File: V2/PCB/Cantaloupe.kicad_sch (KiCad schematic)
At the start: 124 parts, among them J1 USB_In, J2 OLED, J3 Link, J4 Debug, J5 Trackball, J6 Trackpad, Q1 2N7002, Q2 AO3401A, SW1 MX, SW10 MX, SW11 MX, SW12 MX, SW13 MX, SW14 MX, SW15 MX, SW16 MX, SW17 MX, SW18 MX, SW19 MX, SW2 MX, SW20 MX, SW21 MX, SW22 MX, SW23 MX, SW24 MX, SW25 MX, SW26 MX, SW27 MX, SW28 MX, SW29 MX, SW3 MX, SW30 MX, SW31 Encoder, SW32 MX, SW4 MX, SW5 MX, SW6 MX, SW7 MX, SW8 MX, SW9 MX, U1 STM32F4x1CxUx, U2 SRV0504, U3 SRV0504, U4 XC6206P332MR, U5 LMV321, Y1 8MHz

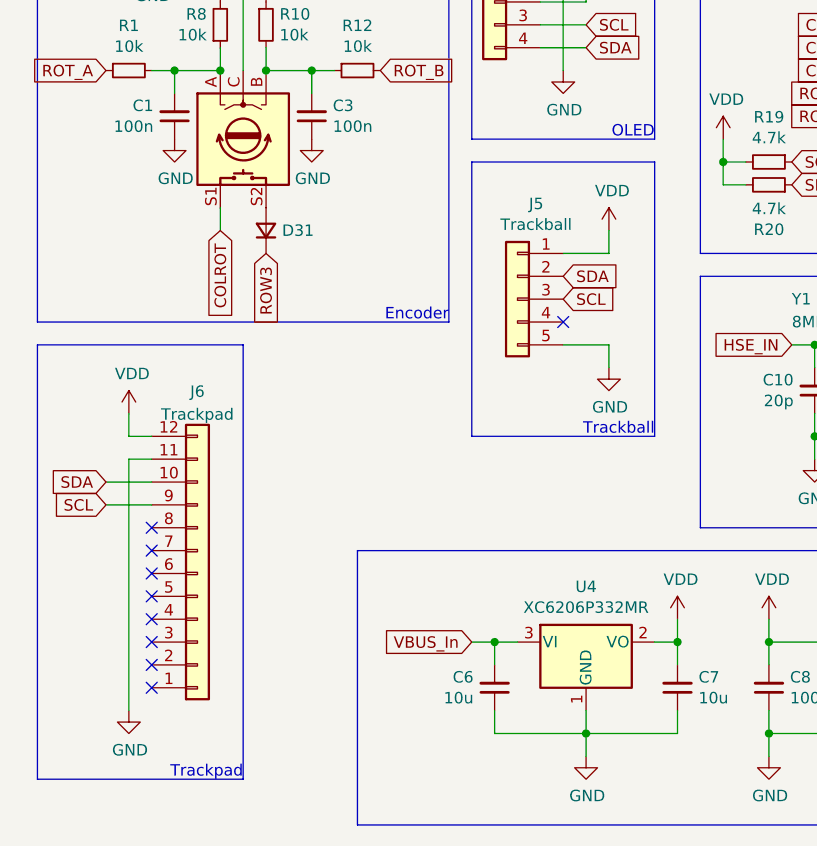
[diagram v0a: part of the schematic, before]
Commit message: Update to V2.1
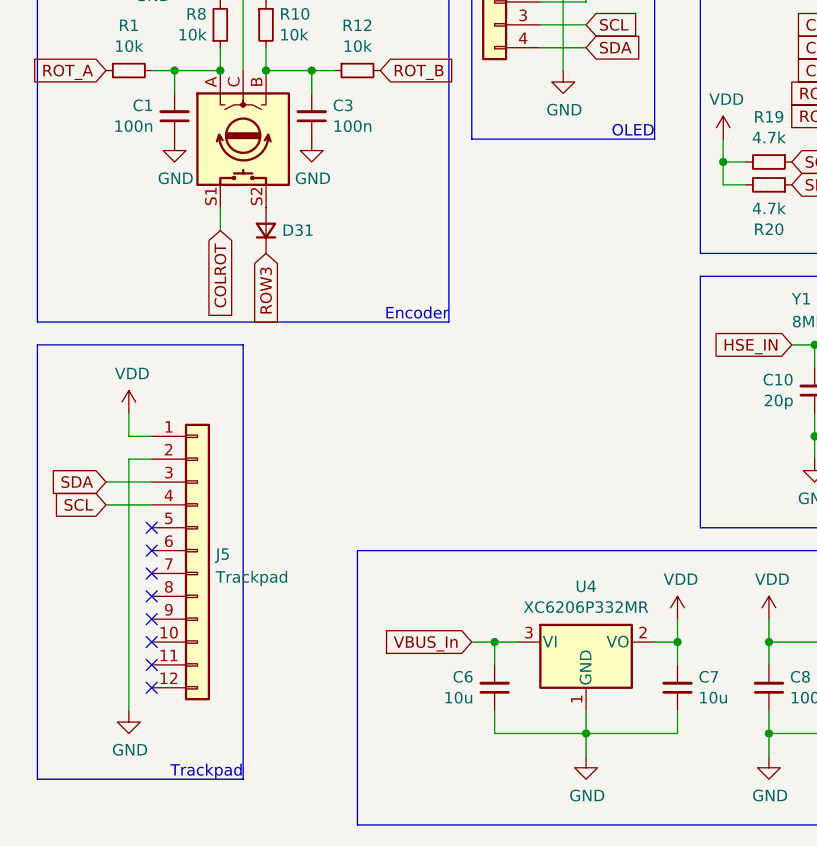
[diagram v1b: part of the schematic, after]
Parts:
- removed J5: Trackball, Ariamelon:pimoroni_trackball_flippable, symbol Connector_Generic:Conn_01x05
- J5: renamed from J6; footprint Ariamelon:FPC-SMD_FPC05012-09200-.5mm-rev -> Connector_FFC-FPC:Hirose_FH12-12S-0.5SH_1x12-1MP_P0.50mm_Horizontal
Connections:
- net GND: now also J5.2 (Pin_2); no longer J5.11 (Pin_11)
- net SCL: now also J5.4 (Pin_4); no longer J5.9 (Pin_9)
- net SDA: now also J5.3 (Pin_3); no longer J5.10 (Pin_10)
- net VDD: now also J5.1 (Pin_1); no longer J5.12 (Pin_12)
- no-connect marks 27 -> 26
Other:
- note removed: "Trackball"
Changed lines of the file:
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@@
   (no_connect (at 30.48 160.02))
   (no_connect (at 109.22 58.42))
-  (no_connect (at 76.2 121.92))
   (no_connect (at 30.48 147.32))
   (no_connect (at 190.5 55.88))
@@
     (stroke (width 0) (type default) (color 0 0 0 0))
   )
-  (wire (pts (xy 81.28 114.3) (xy 81.28 111.76))
-    (stroke (width 0) (type default) (color 0 0 0 0))
-  )
   (polyline (pts (xy 200.66 15.24) (xy 200.66 71.12))
     (stroke (width 0) (type default) (color 0 0 0 0))
@@
     (stroke (width 0) (type default) (color 0 0 0 0))
   )
-  (polyline (pts (xy 86.36 104.14) (xy 66.04 104.14))
-    (stroke (width 0) (type default) (color 0 0 0 0))
-  )
   (wire (pts (xy 38.1 22.86) (xy 38.1 25.4))
     (stroke (width 0) (type default) (color 0 0 0 0))
@@
     (stroke (width 0) (type default) (color 0 0 0 0))
   )
-  (polyline (pts (xy 66.04 134.62) (xy 86.36 134.62))
-    (stroke (width 0) (type default) (color 0 0 0 0))
-  )
   (wire (pts (xy 129.54 165.1) (xy 129.54 167.64))
     (stroke (width 0) (type default) (color 0 0 0 0))
@@
     (stroke (width 0) (type default) (color 0 0 0 0))
   )
-  (wire (pts (xy 81.28 124.46) (xy 76.2 124.46))
-    (stroke (width 0) (type default) (color 0 0 0 0))
-  )
   (polyline (pts (xy 134.62 116.84) (xy 134.62 144.78))
     (stroke (width 0) (type default) (color 0 0 0 0))
@@
     (stroke (width 0) (type default) (color 0 0 0 0))
   )
-  (polyline (pts (xy 66.04 104.14) (xy 66.04 134.62))
-    (stroke (width 0) (type default) (color 0 0 0 0))
-  )
   (wire (pts (xy 60.96 35.56) (xy 58.42 35.56))
     (stroke (width 0) (type default) (color 0 0 0 0))
@@
     (stroke (width 0) (type default) (color 0 0 0 0))
   )
-  (polyline (pts (xy 86.36 134.62) (xy 86.36 104.14))
-    (stroke (width 0) (type default) (color 0 0 0 0))
-  )
   (wire (pts (xy 68.58 157.48) (xy 71.12 157.48))
     (stroke (width 0) (type default) (color 0 0 0 0))
@@
     (stroke (width 0) (type default) (color 0 0 0 0))
   )
-  (wire (pts (xy 81.28 127) (xy 81.28 124.46))
-    (stroke (width 0) (type default) (color 0 0 0 0))
-  )
   (wire (pts (xy 96.52 106.68) (xy 93.98 106.68))
     (stroke (width 0) (type default) (color 0 0 0 0))
@@
     (stroke (width 0) (type default) (color 0 0 0 0))
   )
-  (wire (pts (xy 76.2 114.3) (xy 81.28 114.3))
-    (stroke (width 0) (type default) (color 0 0 0 0))
-  )
   (wire (pts (xy 76.2 71.12) (xy 66.04 71.12))
     (stroke (width 0) (type default) (color 0 0 0 0))
@@
     (effects (font (size 1.27 1.27)) (justify right bottom))
   )
-  (text "Trackball" (at 86.36 134.62 180)
-    (effects (font (size 1.27 1.27)) (justify right bottom))
-  )
   (global_label "D-" (shape input) (at 170.18 91.44 180) (fields_autoplaced)
     (effects (font (size 1.27 1.27)) (justify right))
@@
     )
   )
-  (global_label "SCL" (shape input) (at 76.2 119.38 0) (fields_autoplaced)
-    (effects (font (size 1.27 1.27)) (justify left))
-    (property "Intersheet References" "${INTERSHEET_REFS}" (id 0) (at 0 0 0)
-      (effects (font (size 1.27 1.27)) hide)
-    )
-  )
   (global_label "ROW1" (shape input) (at 25.4 40.64 180) (fields_autoplaced)
     (effects (font (size 1.27 1.27)) (justify right))
@@
     )
   )
-  (global_label "SDA" (shape input) (at 76.2 116.84 0) (fields_autoplaced)
-    (effects (font (size 1.27 1.27)) (justify left))
-    (property "Intersheet References" "${INTERSHEET_REFS}" (id 0) (at 0 0 0)
-      (effects (font (size 1.27 1.27)) hide)
-    )
-  )
   (global_label "SDA" (shape input) (at 109.22 81.28 180) (fields_autoplaced)
     (effects (font (size 1.27 1.27)) (justify right))
@@
     (pin "1")
   )
-  (symbol (lib_id "Connector_Generic:Conn_01x05") (at 71.12 119.38 0) (mirror y) (unit 1)
-    (in_bom yes) (on_board yes)
-    (property "Reference" "J5" (id 0) (at 73.2028 108.7882 0))
-    (property "Value" "Trackball" (id 1) (at 73.2028 111.0996 0))
-    (property "Footprint" "Ariamelon:pimoroni_trackball_flippable" (id 2) (at 71.12 119.38 0)
-      (effects (font (size 1.27 1.27)) hide)
-    )
-    (property "Datasheet" "~" (id 3) (at 71.12 119.38 0)
-      (effects (font (size 1.27 1.27)) hide)
-    )
-    (pin "1")
-    (pin "2")
-    (pin "3")
-    (pin "4")
-    (pin "5")
-  )
-  (symbol (lib_id "power:VDD") (at 81.28 111.76 0) (unit 1)
-    (in_bom yes) (on_board yes)
-    (property "Reference" "#PWR0130" (id 0) (at 81.28 115.57 0)
-      (effects (font (size 1.27 1.27)) hide)
-    )
-    (property "Value" "VDD" (id 1) (at 81.661 107.3658 0))
-    (property "Footprint" "" (id 2) (at 81.28 111.76 0)
-      (effects (font (size 1.27 1.27)) hide)
-    )
-    (property "Datasheet" "" (id 3) (at 81.28 111.76 0)
-      (effects (font (size 1.27 1.27)) hide)
-    )
-    (pin "1")
-  )
   (symbol (lib_id "Device:R_Small") (at 182.88 144.78 0) (unit 1)
     (in_bom yes) (on_board yes)
@@
     (pin "1")
   )
-  (symbol (lib_id "power:GND") (at 81.28 127 0) (unit 1)
-    (in_bom yes) (on_board yes)
-    (property "Reference" "#PWR0131" (id 0) (at 81.28 133.35 0)
-      (effects (font (size 1.27 1.27)) hide)
-    )
-    (property "Value" "GND" (id 1) (at 81.407 131.3942 0))
-    (property "Footprint" "" (id 2) (at 81.28 127 0)
-      (effects (font (size 1.27 1.27)) hide)
-    )
-    (property "Datasheet" "" (id 3) (at 81.28 127 0)
-      (effects (font (size 1.27 1.27)) hide)
-    )
-    (pin "1")
-  )
   (symbol (lib_id "power:GND") (at 152.4 137.16 0) (mirror y) (unit 1)
     (in_bom yes) (on_board yes)
@@
     (pin "1")
   )
-  (symbol (lib_id "Connector_Generic:Conn_01x12") (at 35.56 149.86 0) (mirror x) (unit 1)
+  (symbol (lib_id "Connector_Generic:Conn_01x12") (at 35.56 147.32 0) (unit 1)
     (in_bom yes) (on_board yes) (fields_autoplaced)
-    (property "Reference" "J6" (id 0) (at 35.56 129.6502 0))
-    (property "Value" "Trackpad" (id 1) (at 35.56 132.1871 0))
-    (property "Footprint" "Ariamelon:FPC-SMD_FPC05012-09200-.5mm-rev" (id 2) (at 35.56 149.86 0)
+    (property "Reference" "J5" (id 0) (at 37.592 147.7553 0)
+      (effects (font (size 1.27 1.27)) (justify left))
+    )
+    (property "Value" "Trackpad" (id 1) (at 37.592 150.2922 0)
+      (effects (font (size 1.27 1.27)) (justify left))
+    )
+    (property "Footprint" "Connector_FFC-FPC:Hirose_FH12-12S-0.5SH_1x12-1MP_P0.50mm_Horizontal" (id 2) (at 35.56 147.32 0)
       (effects (font (size 1.27 1.27)) hide)
     )
-    (property "Datasheet" "~" (id 3) (at 35.56 149.86 0)
+    (property "Datasheet" "~" (id 3) (at 35.56 147.32 0)
       (effects (font (size 1.27 1.27)) hide)
     )
@@
       (reference "#PWR0129") (unit 1) (value "VDD") (footprint "")
     )
-    (path "/00000000-0000-0000-0000-0000624bb1ab"
-      (reference "#PWR0130") (unit 1) (value "VDD") (footprint "")
-    )
-    (path "/00000000-0000-0000-0000-0000625e0542"
-      (reference "#PWR0131") (unit 1) (value "GND") (footprint "")
-    )
     (path "/00000000-0000-0000-0000-0000624b93cd"
       (reference "#PWR0132") (unit 1) (value "VDD") (footprint "")
@@
       (reference "J4") (unit 1) (value "Debug") (footprint "Ariamelon:Debug_JTAG_SWD")
     )
-    (path "/00000000-0000-0000-0000-0000624ba1a7"
-      (reference "J5") (unit 1) (value "Trackball") (footprint "Ariamelon:pimoroni_trackball_flippable")
-    )
     (path "/5619f808-0333-40cf-b4ec-f3a4ff626417"
-      (reference "J6") (unit 1) (value "Trackpad") (footprint "Ariamelon:FPC-SMD_FPC05012-09200-.5mm-rev")
+      (reference "J5") (unit 1) (value "Trackpad") (footprint "Connector_FFC-FPC:Hirose_FH12-12S-0.5SH_1x12-1MP_P0.50mm_Horizontal")
     )
     (path "/00000000-0000-0000-0000-00006217adb6"
